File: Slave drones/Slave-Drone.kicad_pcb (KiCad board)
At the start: 4 copper layers, 32 x 32 mm, 46 parts, among them J1 Conn_01x02, J2 Conn_01x02, J3 Conn_01x02, J4 Conn_01x02, J5 USB_C_Receptacle_USB2.0_16P, J6 Conn_01x02, SW1 SW_Push, SW2 SW_Push, U1 MPU6500, U2 QMC5883L, U3 ESP32-S3-MINI-1, U4 AP2112K-3.3

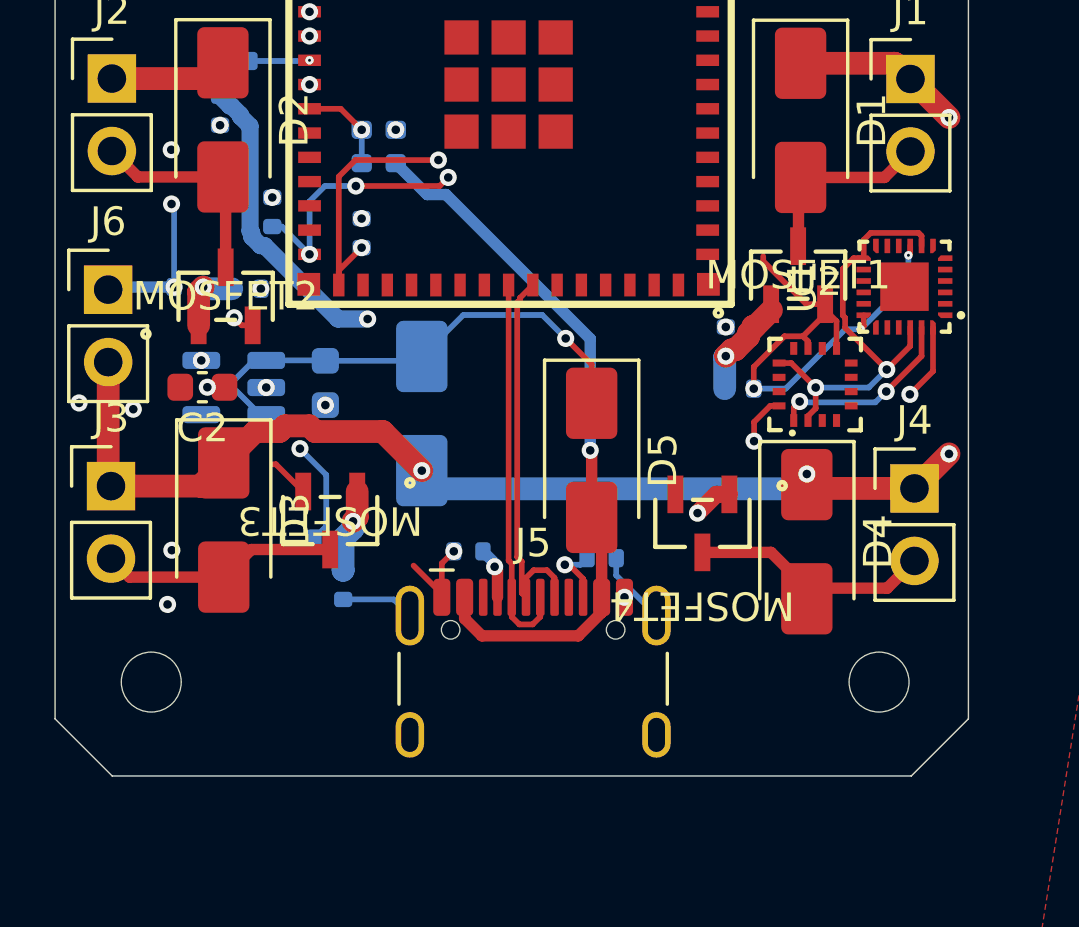
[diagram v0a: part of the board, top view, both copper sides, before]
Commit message: corrected mosfet placement
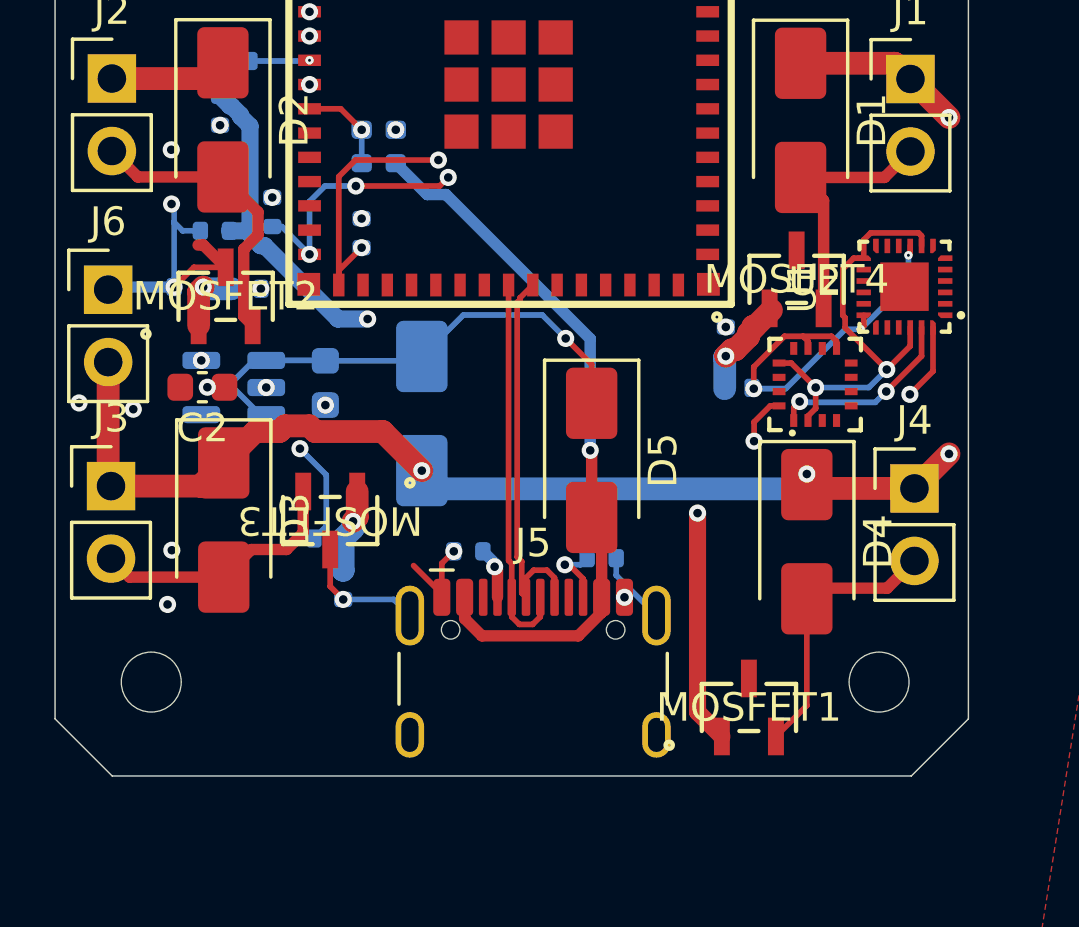
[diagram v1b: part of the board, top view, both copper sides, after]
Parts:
- added R4: 10K, Resistor_SMD:R_0402_1005Metric, B.Cu at (122.3, 82.4)
- moved R1 19.2 mm to (104.0, 76.9), turned to 180 degrees
- moved MOSFET1 15.2 mm to (122.7, 93.6)
- moved MOSFET4 9.17 mm to (124.4, 78.6), turned to 0 degrees
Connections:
- MOSFET1 pad 1: /Motor4 -> /Motor3
- MOSFET1 pad 2: GND -> Net-(D4-A)
- MOSFET1 pad 3: Net-(D1-A) -> GND
- MOSFET2 pad 2: GND -> Net-(D2-A)
- MOSFET2 pad 3: Net-(D2-A) -> GND
- MOSFET3 pad 2: GND -> Net-(D3-A)
- MOSFET3 pad 3: Net-(D3-A) -> GND
- MOSFET4 pad 1: /Motor3 -> /Motor4
- MOSFET4 pad 2: GND -> Net-(D1-A)
- MOSFET4 pad 3: Net-(D4-A) -> GND
- R1 pad 1: /Motor4 -> /Motor3
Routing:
- net /Motor3: track 27.7 -> 35.2 mm
- net Net-(D2-A): track 7.47 -> 10.3 mm
- net GND: track 42.5 -> 39.7 mm
- net Net-(D1-A): track 6.88 -> 9.58 mm
- net Net-(D4-A): track 8.34 -> 9.44 mm
- net Net-(D3-A): track 8.35 -> 9.09 mm

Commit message: nothing
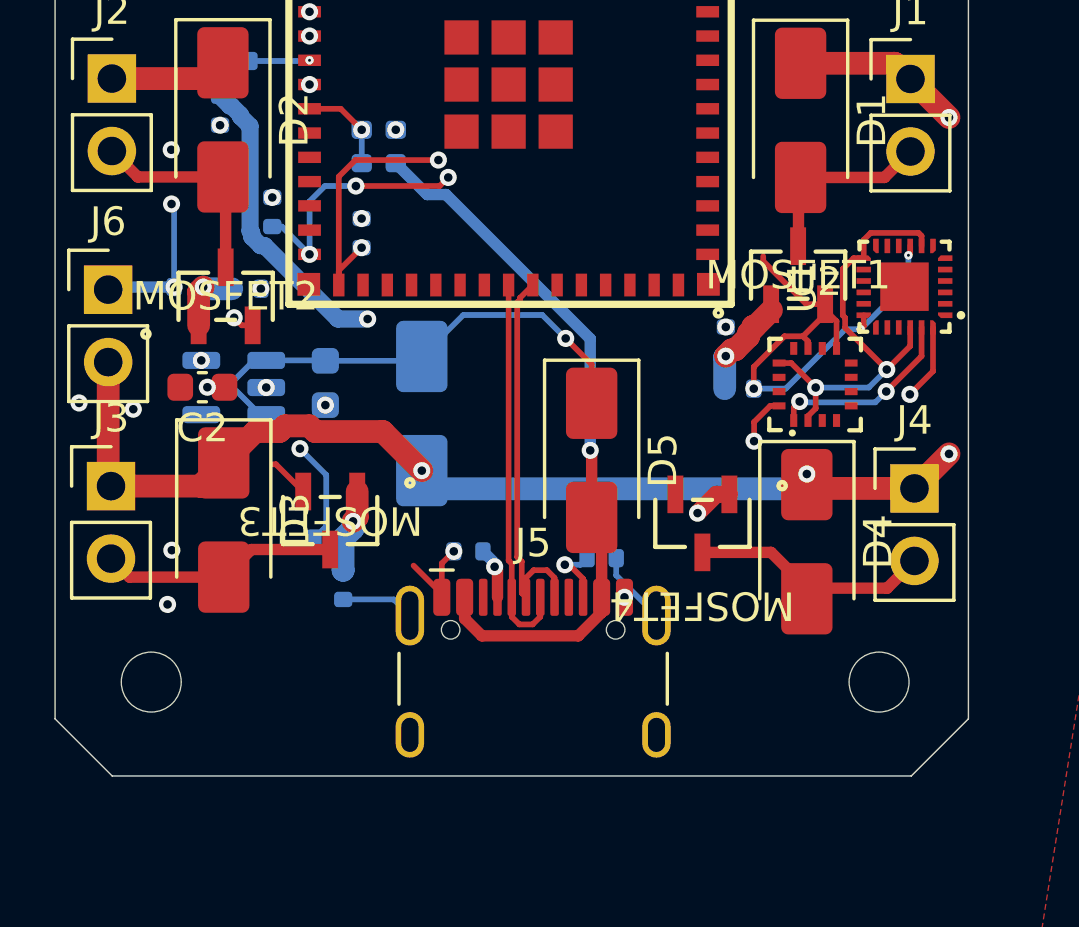
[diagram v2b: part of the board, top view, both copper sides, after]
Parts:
- removed the R4 at (122.3, 82.4)
- moved R1 19.2 mm to (122.4, 82.4), turned to 0 degrees
- moved MOSFET1 15.2 mm to (124.4, 78.5)
- moved MOSFET4 9.17 mm to (121.1, 87.2), turned to 180 degrees
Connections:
- MOSFET1 pad 1: /Motor3 -> /Motor4
- MOSFET1 pad 2: Net-(D4-A) -> GND
- MOSFET1 pad 3: GND -> Net-(D1-A)
- MOSFET2 pad 2: Net-(D2-A) -> GND
- MOSFET2 pad 3: GND -> Net-(D2-A)
- MOSFET3 pad 2: Net-(D3-A) -> GND
- MOSFET3 pad 3: GND -> Net-(D3-A)
- MOSFET4 pad 1: /Motor4 -> /Motor3
- MOSFET4 pad 2: Net-(D1-A) -> GND
- MOSFET4 pad 3: GND -> Net-(D4-A)
- R1 pad 1: /Motor3 -> /Motor4
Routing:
- net /Motor3: track 35.2 -> 27.7 mm
- net Net-(D2-A): track 10.3 -> 7.47 mm
- net GND: track 39.7 -> 42.5 mm
- net Net-(D1-A): track 9.58 -> 6.88 mm
- net Net-(D4-A): track 9.44 -> 8.34 mm
- net Net-(D3-A): track 9.09 -> 8.35 mm
